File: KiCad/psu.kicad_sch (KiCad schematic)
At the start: 23 parts, among them J8 Screw_Terminal_01x03, J9 PSU ground, J9 Screw_Terminal_01x01

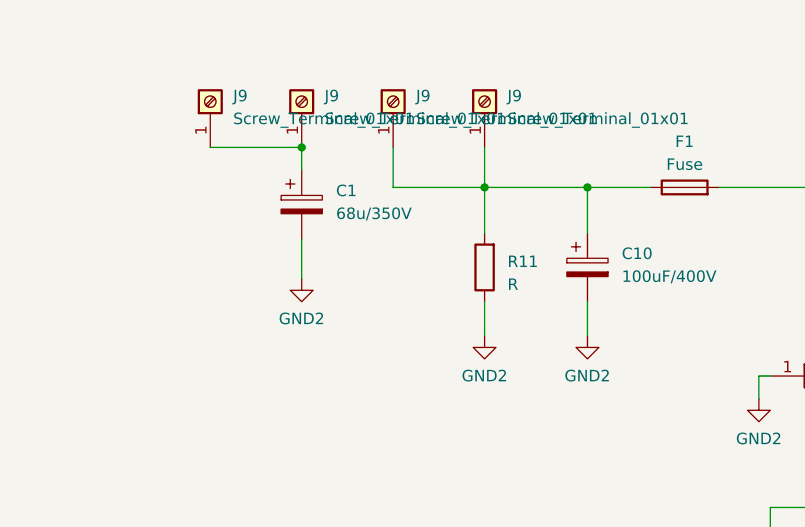
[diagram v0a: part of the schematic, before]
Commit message: Add files via upload
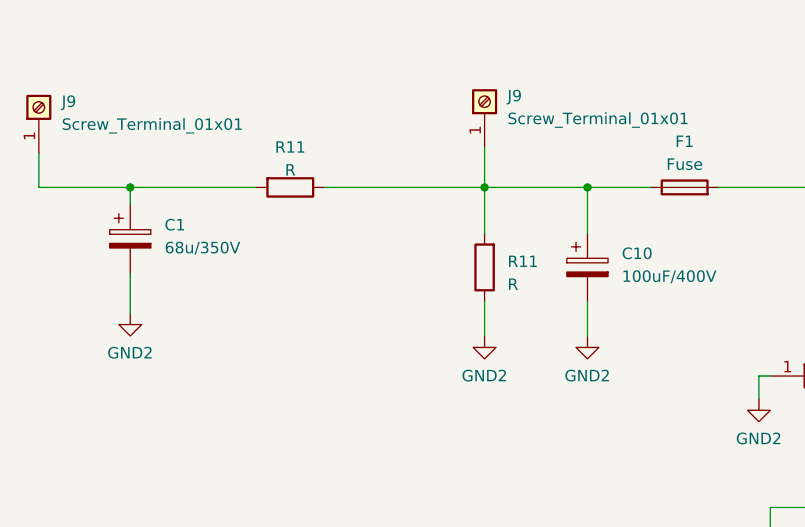
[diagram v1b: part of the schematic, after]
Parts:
- removed J9 (x2): Screw_Terminal_01x01, Connector_Pin:Pin_D1.1mm_L8.5mm_W2.5mm_FlatFork, symbol Connector:Screw_Terminal_01x01
- added R11: R, Resistor_THT:R_Axial_DIN0617_L17.0mm_D6.0mm_P25.40mm_Horizontal, symbol Device:R
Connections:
- net at C10.1, F1.1, J9.1 (Pin_1)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: now also R11.1
- net at C1.1, J9.1 (Pin_1): now also R11.2
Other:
- moved on the sheet: C1, J9
